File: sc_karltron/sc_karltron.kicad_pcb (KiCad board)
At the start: 2 copper layers, 88.6 x 50.6 mm, 6 parts, among them J1 Conn_01x02, J2 Conn_01x02

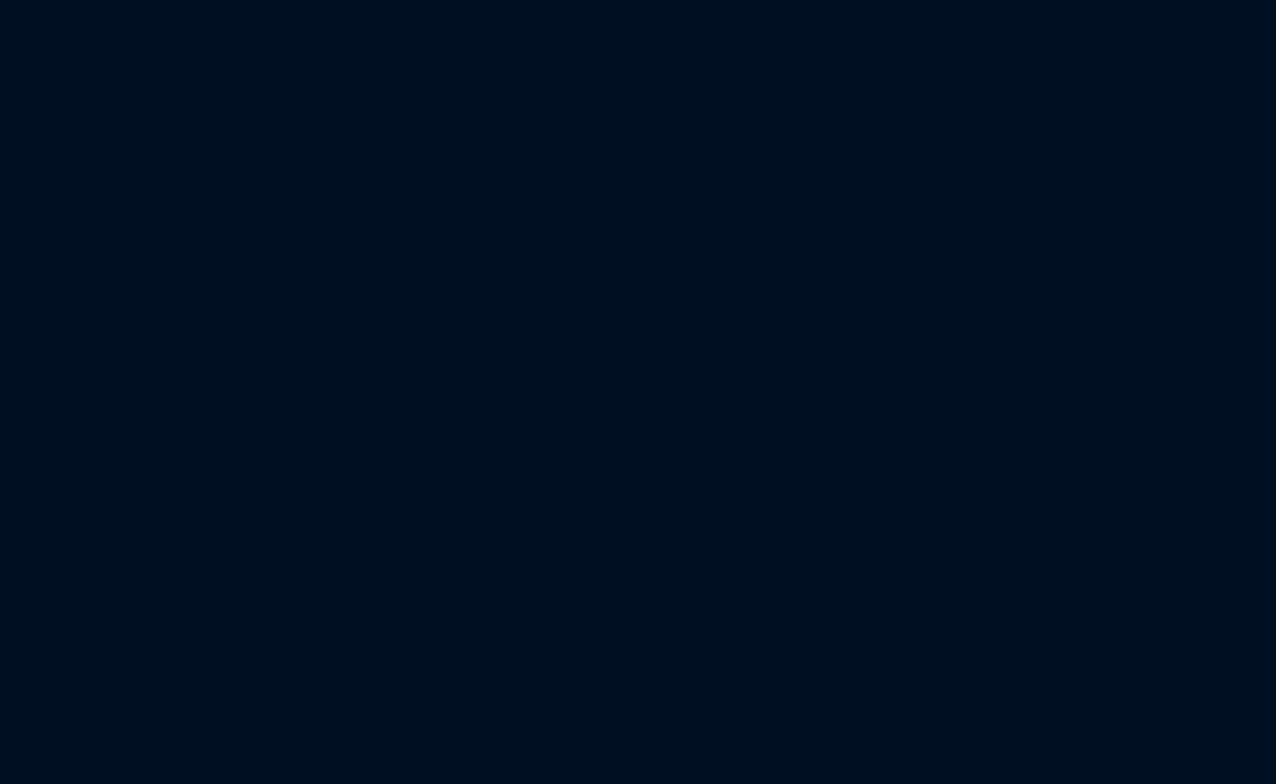
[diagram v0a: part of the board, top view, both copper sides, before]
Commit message: basic components
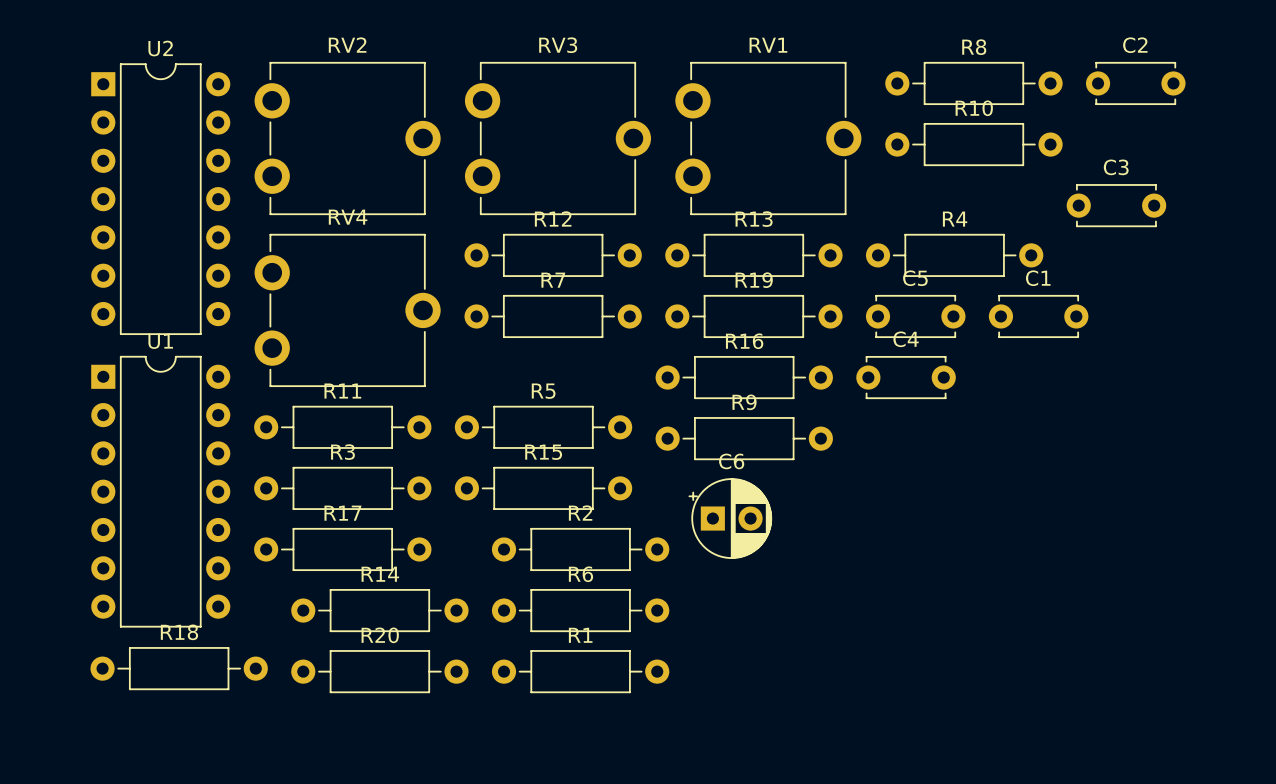
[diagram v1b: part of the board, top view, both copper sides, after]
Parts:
- added C1: C, Capacitor_THT:C_Disc_D5.0mm_W2.5mm_P5.00mm, F.Cu at (171.6, 25.9)
- added C2: C, Capacitor_THT:C_Disc_D5.0mm_W2.5mm_P5.00mm, F.Cu at (178.0, 10.4)
- added C3: C, Capacitor_THT:C_Disc_D5.0mm_W2.5mm_P5.00mm, F.Cu at (176.8, 18.6)
- added C4: C, Capacitor_THT:C_Disc_D5.0mm_W2.5mm_P5.00mm, F.Cu at (162.8, 29.9)
- added C5: C, Capacitor_THT:C_Disc_D5.0mm_W2.5mm_P5.00mm, F.Cu at (163.4, 25.9)
- added C6: C_Polarized, Capacitor_THT:CP_Radial_D5.0mm_P2.50mm, F.Cu at (152.5, 39.3)
- added R1: 100K, Resistor_THT:R_Axial_DIN0207_L6.3mm_D2.5mm_P10.16mm_Horizontal, F.Cu at (138.7, 49.5)
- added R10: 100K, Resistor_THT:R_Axial_DIN0207_L6.3mm_D2.5mm_P10.16mm_Horizontal, F.Cu at (164.7, 14.5)
- added R11: LDR, Resistor_THT:R_Axial_DIN0207_L6.3mm_D2.5mm_P10.16mm_Horizontal, F.Cu at (122.9, 33.2)
- added R12: 10K, Resistor_THT:R_Axial_DIN0207_L6.3mm_D2.5mm_P10.16mm_Horizontal, F.Cu at (136.8, 21.9)
- added R13: 100K, Resistor_THT:R_Axial_DIN0207_L6.3mm_D2.5mm_P10.16mm_Horizontal, F.Cu at (150.1, 21.9)
- added R14: 10K, Resistor_THT:R_Axial_DIN0207_L6.3mm_D2.5mm_P10.16mm_Horizontal, F.Cu at (125.3, 45.4)
- added R15: 100K, Resistor_THT:R_Axial_DIN0207_L6.3mm_D2.5mm_P10.16mm_Horizontal, F.Cu at (136.2, 37.3)
- added R16: 1M, Resistor_THT:R_Axial_DIN0207_L6.3mm_D2.5mm_P10.16mm_Horizontal, F.Cu at (149.5, 29.9)
- added R17: 100K, Resistor_THT:R_Axial_DIN0207_L6.3mm_D2.5mm_P10.16mm_Horizontal, F.Cu at (122.9, 41.4)
- added R18: 1M, Resistor_THT:R_Axial_DIN0207_L6.3mm_D2.5mm_P10.16mm_Horizontal, F.Cu at (112.0, 49.2)
- added R19: 100K, Resistor_THT:R_Axial_DIN0207_L6.3mm_D2.5mm_P10.16mm_Horizontal, F.Cu at (150.1, 25.9)
- added R2: 100K, Resistor_THT:R_Axial_DIN0207_L6.3mm_D2.5mm_P10.16mm_Horizontal, F.Cu at (138.7, 41.4)
- added R20: 1M, Resistor_THT:R_Axial_DIN0207_L6.3mm_D2.5mm_P10.16mm_Horizontal, F.Cu at (125.3, 49.5)
- added R3: 100K, Resistor_THT:R_Axial_DIN0207_L6.3mm_D2.5mm_P10.16mm_Horizontal, F.Cu at (122.9, 37.3)
- added R4: LDR, Resistor_THT:R_Axial_DIN0207_L6.3mm_D2.5mm_P10.16mm_Horizontal, F.Cu at (163.4, 21.9)
- added R5: 10K, Resistor_THT:R_Axial_DIN0207_L6.3mm_D2.5mm_P10.16mm_Horizontal, F.Cu at (136.2, 33.2)
- added R6: 100K, Resistor_THT:R_Axial_DIN0207_L6.3mm_D2.5mm_P10.16mm_Horizontal, F.Cu at (138.7, 45.4)
- added R7: 10K, Resistor_THT:R_Axial_DIN0207_L6.3mm_D2.5mm_P10.16mm_Horizontal, F.Cu at (136.8, 25.9)
- added R8: LDR, Resistor_THT:R_Axial_DIN0207_L6.3mm_D2.5mm_P10.16mm_Horizontal, F.Cu at (164.7, 10.4)
- added R9: 10K, Resistor_THT:R_Axial_DIN0207_L6.3mm_D2.5mm_P10.16mm_Horizontal, F.Cu at (149.5, 34.0)
- added RV1: B100K, Potentiometer_THT:Potentiometer_ACP_CA9-V10_Vertical, F.Cu at (151.2, 16.6)
- added RV2: B100K, Potentiometer_THT:Potentiometer_ACP_CA9-V10_Vertical, F.Cu at (123.3, 16.6)
- added RV3: B100K, Potentiometer_THT:Potentiometer_ACP_CA9-V10_Vertical, F.Cu at (137.2, 16.6)
- added RV4: B100K, Potentiometer_THT:Potentiometer_ACP_CA9-V10_Vertical, F.Cu at (123.3, 28.0)
- added U1: TL074, Package_DIP:DIP-14_W7.62mm, F.Cu at (112.1, 29.9)
- added U2: TL074, Package_DIP:DIP-14_W7.62mm, F.Cu at (112.1, 10.5)
